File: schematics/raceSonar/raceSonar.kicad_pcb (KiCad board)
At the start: 2 copper layers, 13 parts, among them P1 CONN_01X08, P10 5V, P11 OUT1, P12 OUT2, P2 CONN_02X04, P4 CONN_02X07, P5 CONN_01X10, P6 CONTROL1, P7 CONTROL2, P8 35V, P9 GND, U1 Arduino_Mini, U2 L293D

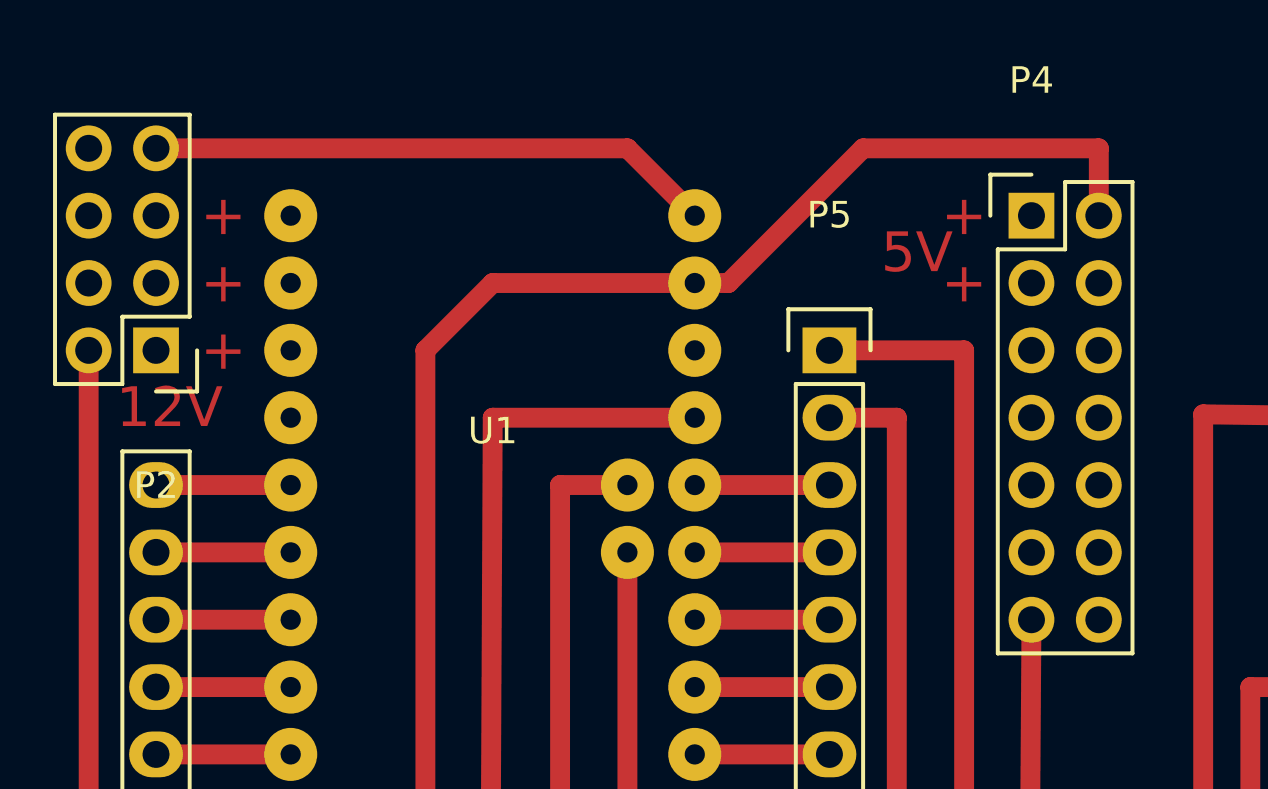
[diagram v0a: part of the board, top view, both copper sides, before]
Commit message: Schematic
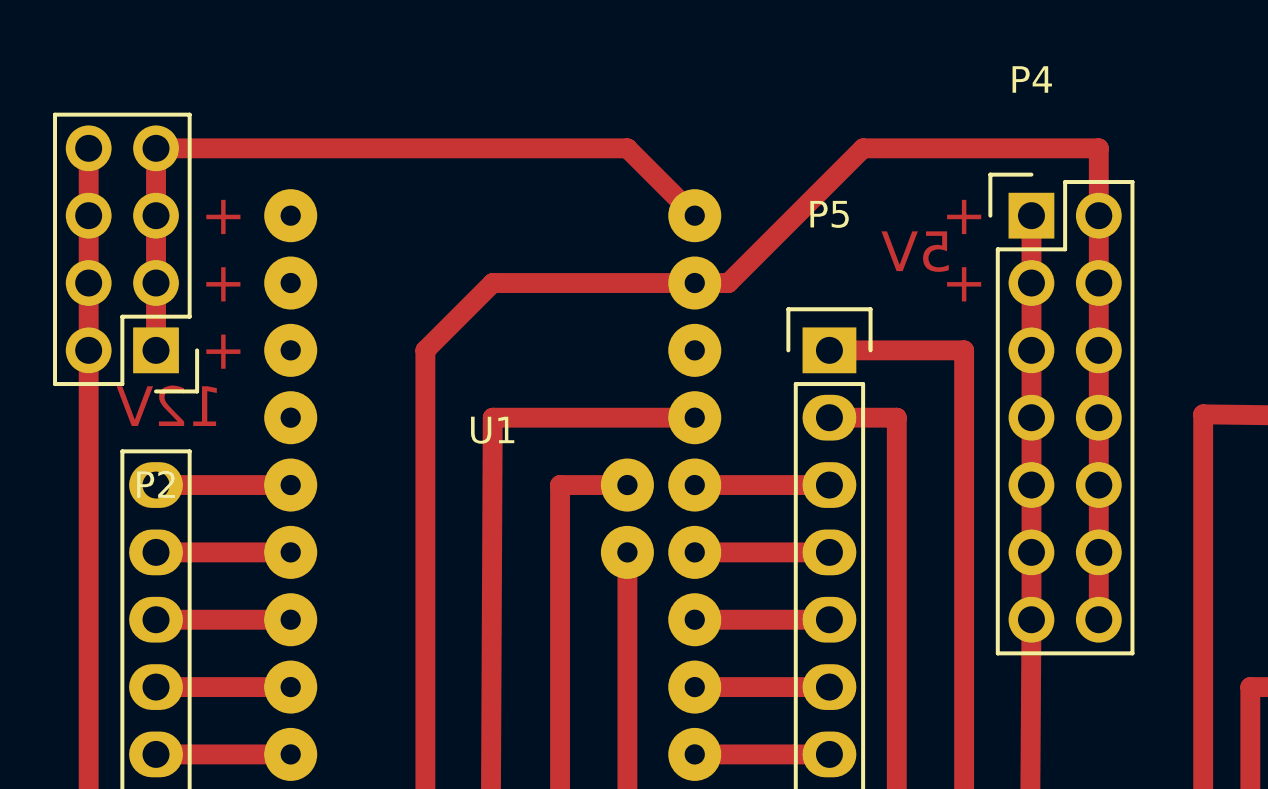
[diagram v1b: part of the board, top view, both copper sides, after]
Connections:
- P2 pad 3: Net-(P2-Pad3) -> Net-(P2-Pad1)
- P2 pad 4: Net-(P2-Pad4) -> Net-(P2-Pad2)
- P2 pad 5: Net-(P2-Pad5) -> Net-(P2-Pad1)
- P2 pad 6: Net-(P2-Pad6) -> Net-(P2-Pad2)
- P2 pad 7: Net-(P2-Pad7) -> Net-(P2-Pad1)
- P2 pad 8: Net-(P2-Pad8) -> Net-(P2-Pad2)
- P4 pad 10: Net-(P4-Pad10) -> Net-(P2-Pad2)
- P4 pad 11: Net-(P4-Pad11) -> Net-(P4-Pad1)
- P4 pad 12: Net-(P4-Pad12) -> Net-(P2-Pad2)
- P4 pad 13: Net-(P4-Pad13) -> Net-(P4-Pad1)
- P4 pad 14: Net-(P4-Pad14) -> Net-(P2-Pad2)
- P4 pad 3: Net-(P4-Pad3) -> Net-(P4-Pad1)
- P4 pad 4: Net-(P4-Pad4) -> Net-(P2-Pad2)
- P4 pad 5: Net-(P4-Pad5) -> Net-(P4-Pad1)
- P4 pad 6: Net-(P4-Pad6) -> Net-(P2-Pad2)
- P4 pad 7: Net-(P4-Pad7) -> Net-(P4-Pad1)
- P4 pad 8: Net-(P4-Pad8) -> Net-(P2-Pad2)
- P4 pad 9: Net-(P4-Pad9) -> Net-(P4-Pad1)
- U1 pad 10: Net-(P4-Pad13) -> Net-(P4-Pad1)
- U1 pad 7: Net-(P2-Pad7) -> Net-(P2-Pad1)
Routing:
- net Net-(P4-Pad1): track 0.00 -> 89.7 mm
- net Net-(P4-Pad13): track 74.4 -> 0.00 mm
- net Net-(P2-Pad1): track 0.00 -> 29.0 mm
- net Net-(P2-Pad2): track 99.7 -> 122.5 mm
- net Net-(P2-Pad7): track 21.4 -> 0.00 mm
